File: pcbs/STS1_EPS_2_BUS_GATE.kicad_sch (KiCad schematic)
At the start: 17 parts, among them Q2 SI7135DP-T1-GE3, Q3 SI7135DP-T1-GE3, Q4 SI7135DP-T1-GE3, Q5 SI7135DP-T1-GE3, U27 TPS2420RSAT

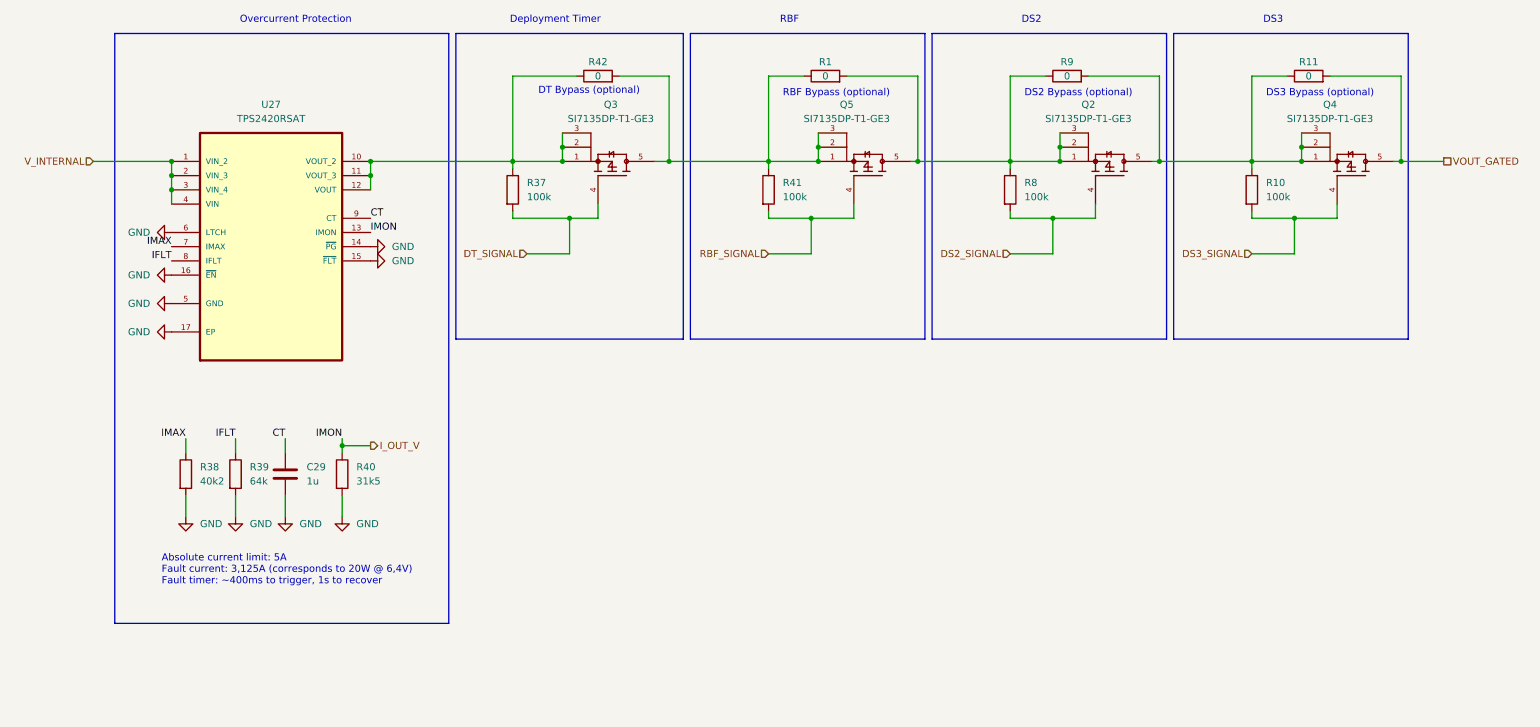
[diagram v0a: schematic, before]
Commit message: worked on sts1_eps_1
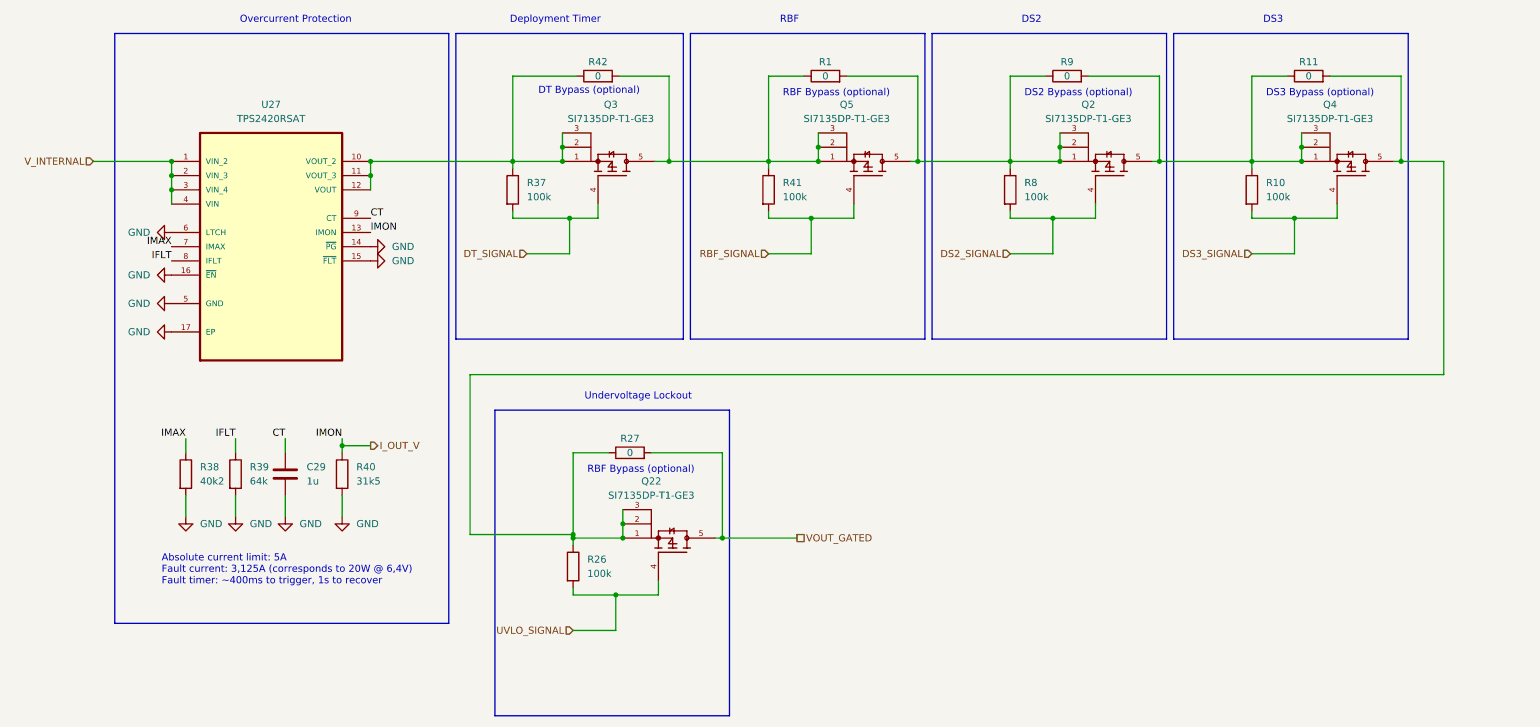
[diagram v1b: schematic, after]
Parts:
- added Q22: SI7135DP-T1-GE3, STS_Package_SO:POWERPAK_SO8_single, symbol STS_Transistor_FET:SI7135DP-T1-GE3
- added R26: 100k, Resistor_SMD:R_0805_2012Metric, symbol Device:R
- added R27: 0, Resistor_SMD:R_0805_2012Metric, symbol Device:R
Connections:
- net VOUT_GATED: now also Q22.5, R27.2; no longer Q4.5, R11.2
- new net: Q22.1, Q22.2, Q22.3, Q4.5, R11.2, R26.1, R27.1
- new net UVLO_SIGNAL: Q22.4, R26.2
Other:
- note added: "Undervoltage Lockout"
